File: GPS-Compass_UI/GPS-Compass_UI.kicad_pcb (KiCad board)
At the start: 2 copper layers, 20 x 95 mm, 28 parts, among them J3 FFC2B28-12-G, SW1 SPDT, SW2 EXT, SW3 RESET, SW4 RESET, SW5 EXT, SW6 EXT, SW7 EXT

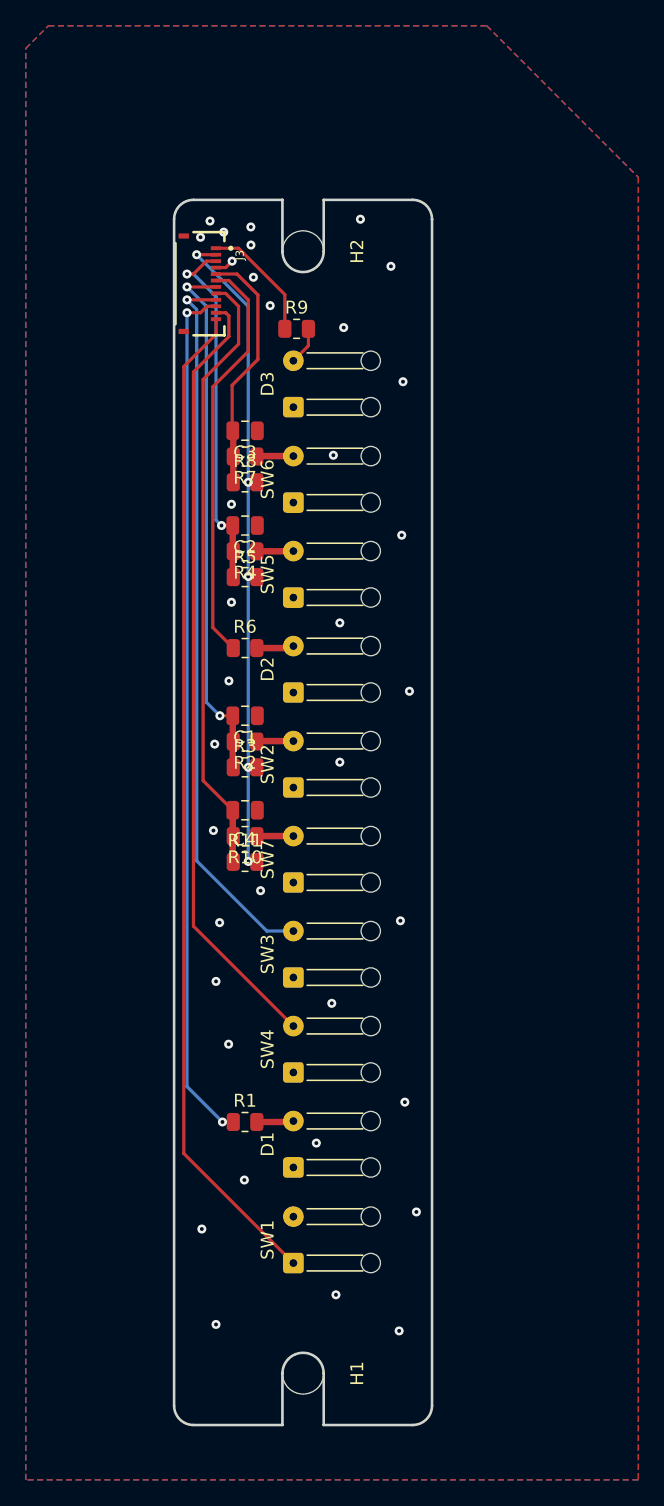
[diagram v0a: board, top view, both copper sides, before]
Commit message: GPS Compass - schematic
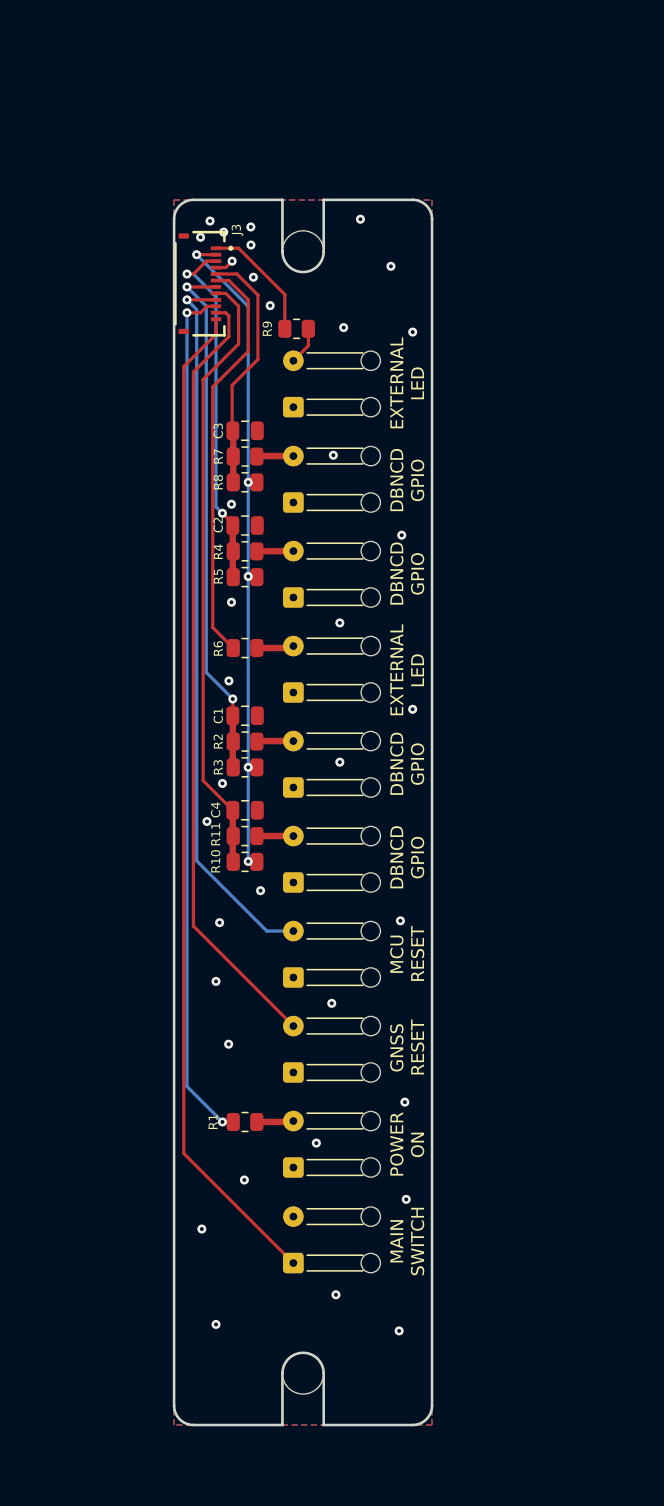
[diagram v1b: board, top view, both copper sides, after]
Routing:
- net /CRD_RST: track 41.6 -> 41.0 mm
- net /EXT0: track 28.5 -> 27.9 mm
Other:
- board text added: "DBNCD GPIO"
- board text added: "EXTERNAL LED"
- board text added: "GNSS RESET"
- board text added: "MAIN SWITCH"
- board text added: "MCU RESET"
- board text added: "POWER ON"

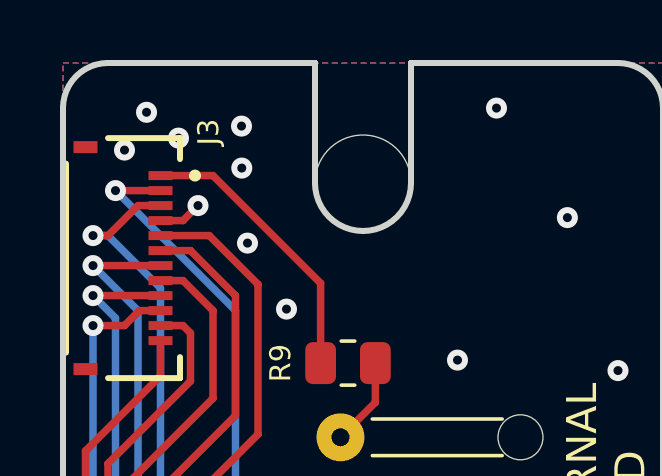
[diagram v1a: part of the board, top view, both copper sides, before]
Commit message: routing
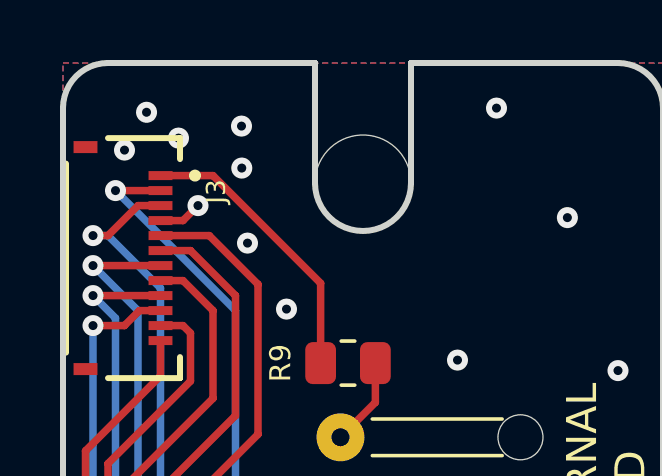
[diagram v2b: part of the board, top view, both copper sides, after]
